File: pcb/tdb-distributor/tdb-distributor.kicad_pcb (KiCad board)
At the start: 2 copper layers, 68 x 68 mm, 55 parts, among them IC1 74HC541D,653, IC2 74HC541D,653, J1 Conn_02x07_Odd_Even, J2 Conn_02x07_Odd_Even, J3 Conn_02x07_Odd_Even, J4 Conn_02x07_Odd_Even, J5 Screw_Terminal_01x03, J6 RJ45_Hanrun_HR911105A_Horizon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, J7 USB_C_Receptacle_USB2.0_16P, J8 Conn_01x02, U1 LM317_TO-220, U2 W5500, U3 R7FA4M1AB3CFM, Y1 25M

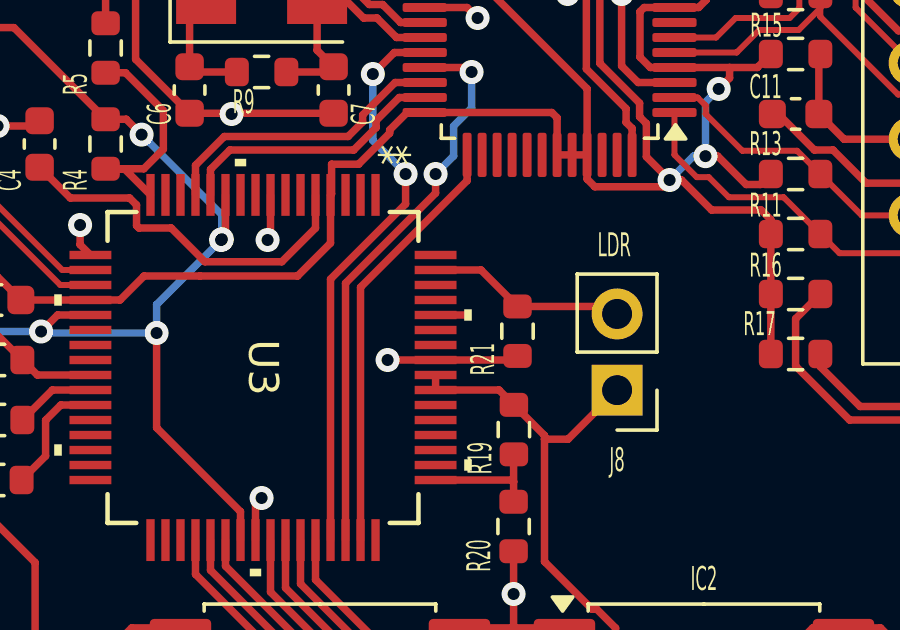
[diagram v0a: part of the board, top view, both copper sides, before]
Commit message: minor drc cleanup
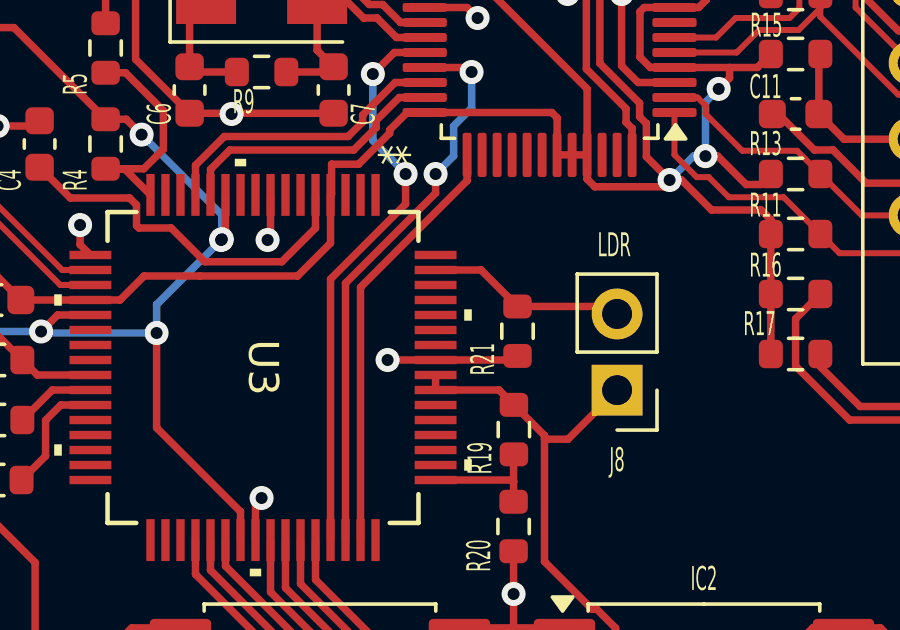
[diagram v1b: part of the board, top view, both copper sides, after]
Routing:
- net unconnected-(U3-P004-Pad60): track 0.96 -> 0.00 mm
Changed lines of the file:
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@@
-	)
-	(segment
-		(start 129.6 38.499874)
-		(end 130.559874 38.499874)
-		(width 0.25)
-		(layer "F.Cu")
-		(net 99)
 	)
 	(segment
